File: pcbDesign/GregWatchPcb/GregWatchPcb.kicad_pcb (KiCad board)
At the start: 2 copper layers, 35 parts, among them J1 AVR-ISP-6, SW1 SW_Push, SW2 SW_Push, SW3 SW_Push, SW4 SW_Push, U1 Nokia_5110_LCD, U2 ATmega328P-AU, U3 74HC14, Y1 16M

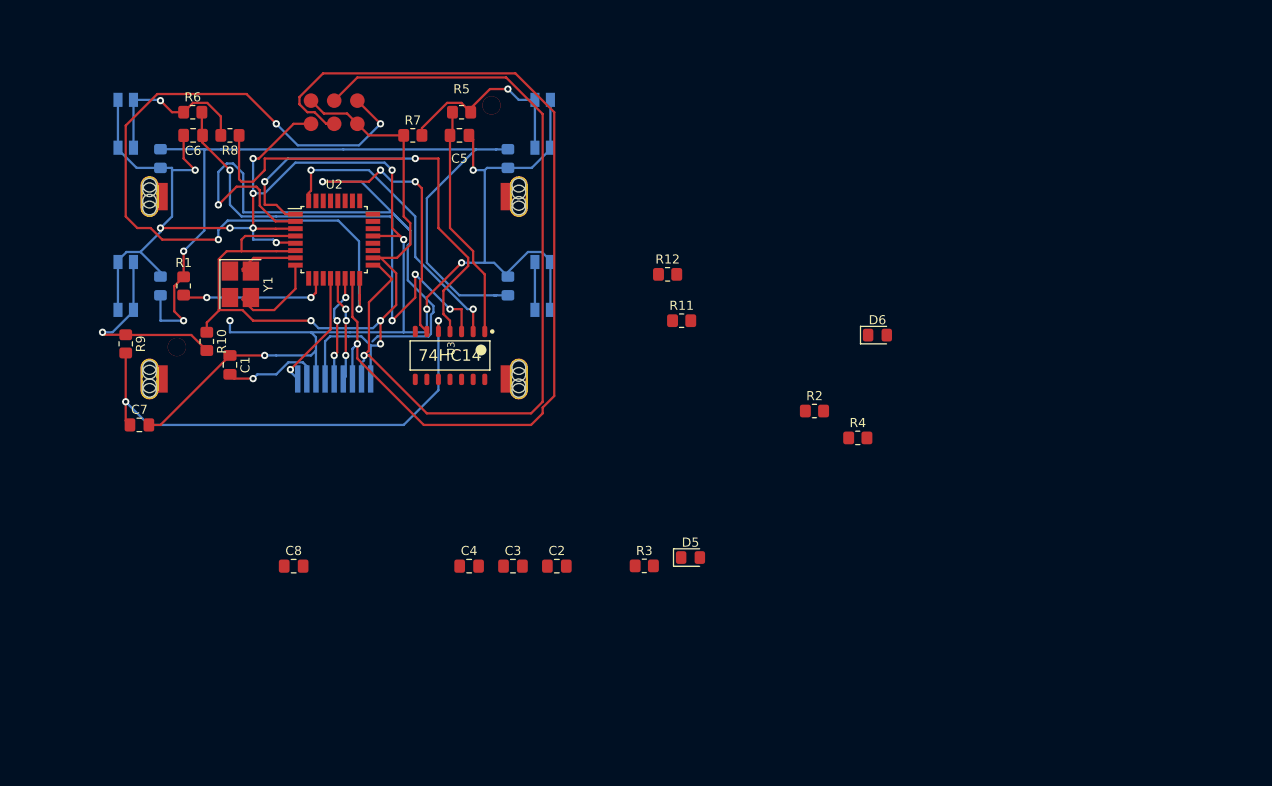
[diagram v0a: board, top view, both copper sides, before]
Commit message: Place and routed the power and IC components
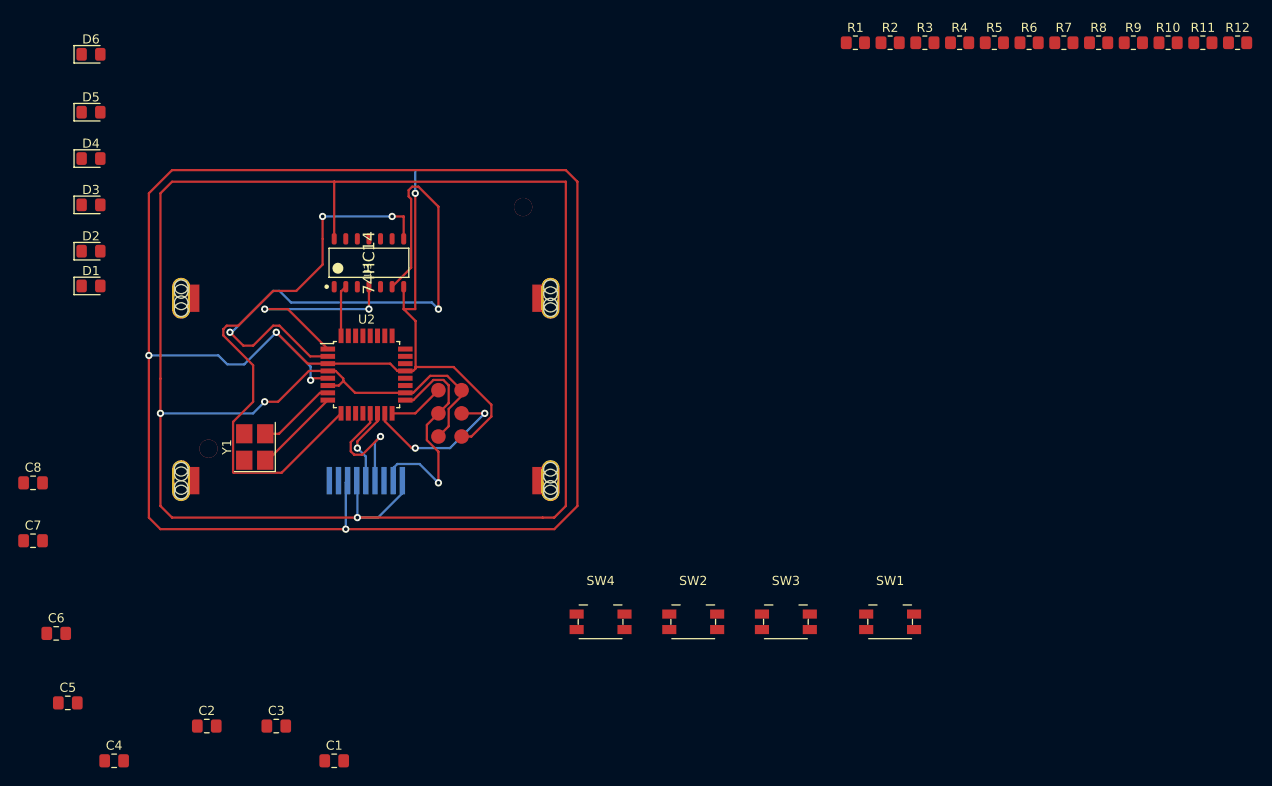
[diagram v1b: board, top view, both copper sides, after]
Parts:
- D1, D2, D3, D4, SW1, SW2, SW3, SW4: moved to F.Cu
- moved R9 115.3 mm to (223.5, 50.8), turned to 0 degrees
- moved R10 110.4 mm to (227.3, 50.8), turned to 0 degrees
- moved R8 95.8 mm to (219.7, 50.8), turned to 0 degrees
- moved R6 92.0 mm to (212.1, 50.8)
- moved D6 91.6 mm to (109.2, 52.1)
- moved SW2 82.8 mm to (175.3, 114.3), turned to 0 degrees
- moved D5 81.9 mm to (109.2, 58.4)
- moved SW3 81.2 mm to (185.4, 114.3), turned to 0 degrees
- moved R1 78.3 mm to (193.0, 50.8), turned to 0 degrees
- moved C5 75.6 mm to (106.7, 123.2)
- moved R7 72.1 mm to (215.9, 50.8)
- moved R12 67.5 mm to (234.9, 50.8)
- moved SW1 66.6 mm to (196.8, 114.3), turned to 0 degrees
- moved R3 65.1 mm to (200.7, 50.8)
- moved R11 64.8 mm to (231.1, 50.8)
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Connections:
- Y1 pad 1: Net-(C2-Pad2) -> Net-(C3-Pad2)
- Y1 pad 2: Net-(C3-Pad2) -> Net-(C2-Pad2)
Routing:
- net +5V: track 122.8 -> 223.7 mm
- net Net-(J1-Pad4): track 106.8 -> 17.2 mm, vias 1 -> 2
- net Net-(D1-Pad2): track 89.3 -> 0.00 mm, vias 2 -> 0
- net Net-(J1-Pad1): track 86.7 -> 6.13 mm, vias 4 -> 0
- net Net-(J1-Pad3): track 94.9 -> 25.5 mm
- net Net-(U2-Pad9): track 0.00 -> 62.9 mm, vias 0 -> 2
- net Net-(C6-Pad1): track 56.3 -> 0.00 mm, vias 4 -> 0
- net Net-(C7-Pad1): track 53.8 -> 0.00 mm, vias 2 -> 0
- net Net-(U2-Pad2): track 102.1 -> 66.3 mm, vias 4 -> 2
- net GND: track 222.5 -> 256.9 mm, vias 14 -> 5
- net Net-(U2-Pad32): track 32.6 -> 5.60 mm, vias 2 -> 0
- net Net-(C5-Pad1): track 25.7 -> 0.00 mm
- net Net-(U2-Pad1): track 48.2 -> 22.6 mm
- net Net-(R10-Pad2): track 22.0 -> 0.00 mm, vias 1 -> 0
- net Net-(R5-Pad1): track 21.8 -> 0.00 mm, vias 1 -> 0
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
